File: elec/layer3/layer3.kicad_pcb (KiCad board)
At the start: 2 copper layers, 125 x 125 mm, 57 parts, among them J10 Conn_01x05, J4 Conn_01x05, J8 XT30PW-M, J9 XT30PW-M, SW1 SW_SPDT_312, SW2 SW_SPDT_312, SW3 SW_SPDT_312, SW4 SW_SPDT_312, U1 CD74HC4067SM, U2 CD74HC4067SM, U4 4754, U5 113991054

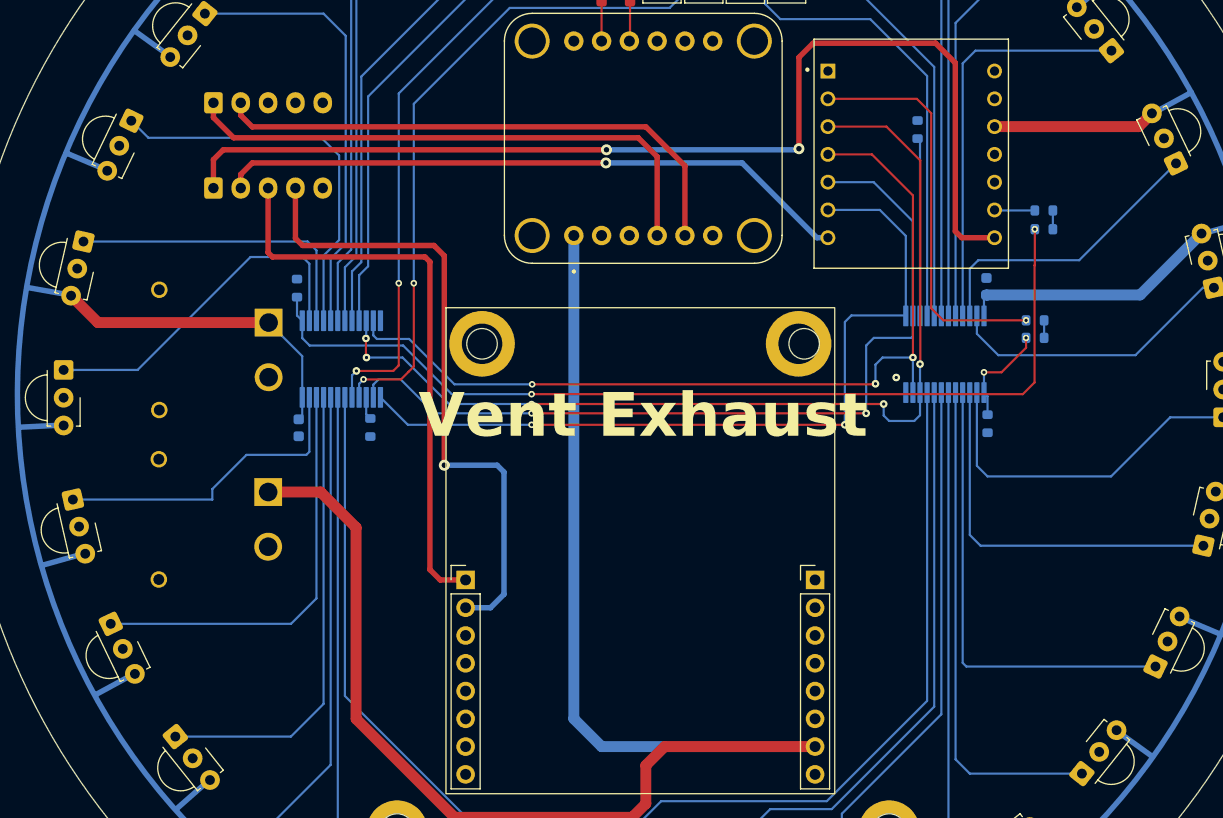
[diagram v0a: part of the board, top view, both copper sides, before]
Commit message: l3 : done
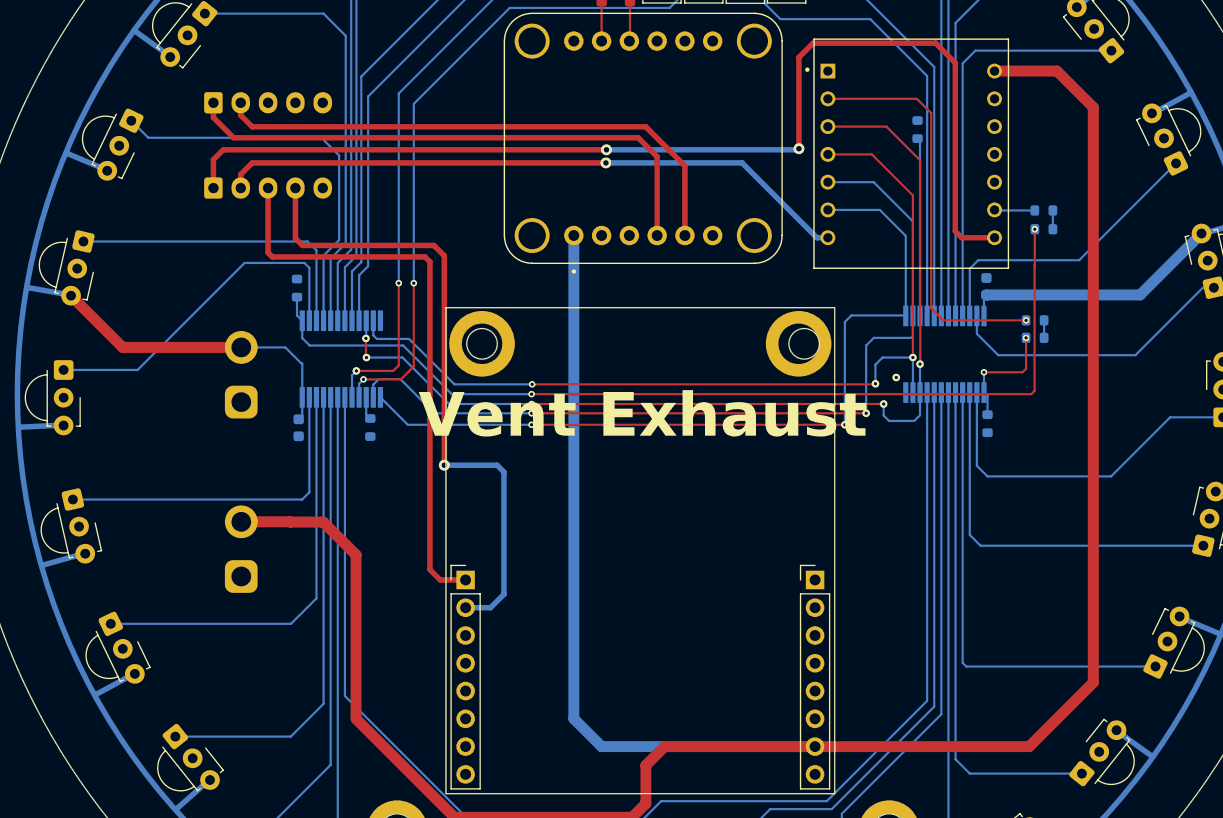
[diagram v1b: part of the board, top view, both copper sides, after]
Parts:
- J8, J9: footprint L3:AMASS_XT30PW-M -> Connector_AMASS:AMASS_XT30UPB-M_1x02_P5.0mm_Vertical
- moved J8 9.18 mm to (109.8, 111.7), turned to 90 degrees
- moved J9 8.89 mm to (109.8, 95.8), turned to 90 degrees
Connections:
- U5 pad 12: +3V3 -> unconnected-(U5-VCC_3V3-Pad12)
- U5 pad 14: unconnected-(U5-VUSB-Pad14) -> +5V
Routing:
- net +5V: track 144.6 -> 235.4 mm
- net +3V3: track 98.6 -> 83.3 mm
- net /IR9: track 29.0 -> 30.6 mm
- net /Mux Com (17-32): track 9.75 -> 10.9 mm
- net /IR8: track 32.2 -> 31.5 mm
